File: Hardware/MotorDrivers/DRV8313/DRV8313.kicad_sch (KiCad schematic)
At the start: 61 parts, among them CN10 PR5L4015-5P-C-F, CN11 PR5L4015-5P-C-F, CN7 PR5L4015-5P-C-F, CN8 PR5L4015-5P-C-F, CN9 PR5L4015-5P-C-F, J1 Conn_01x04_Socket, J3 Conn_01x02_Socket, J4 Conn_01x03_Socket, Q1 BSS123_C427379, Q2 BSS123_C427379, U1 MS8313, U2 TLV9001IDCK, U35 PR5L5015-5P-C-H, U36 PR5L5015-5P-C-H, U37 PR5L5015-5P-C-H, U38 PR5L5015-5P-C-H, U39 PR5L5015-5P-C-H, U5 INA241A2xD, U6 INA241A2xD, U7 INA241A2xD

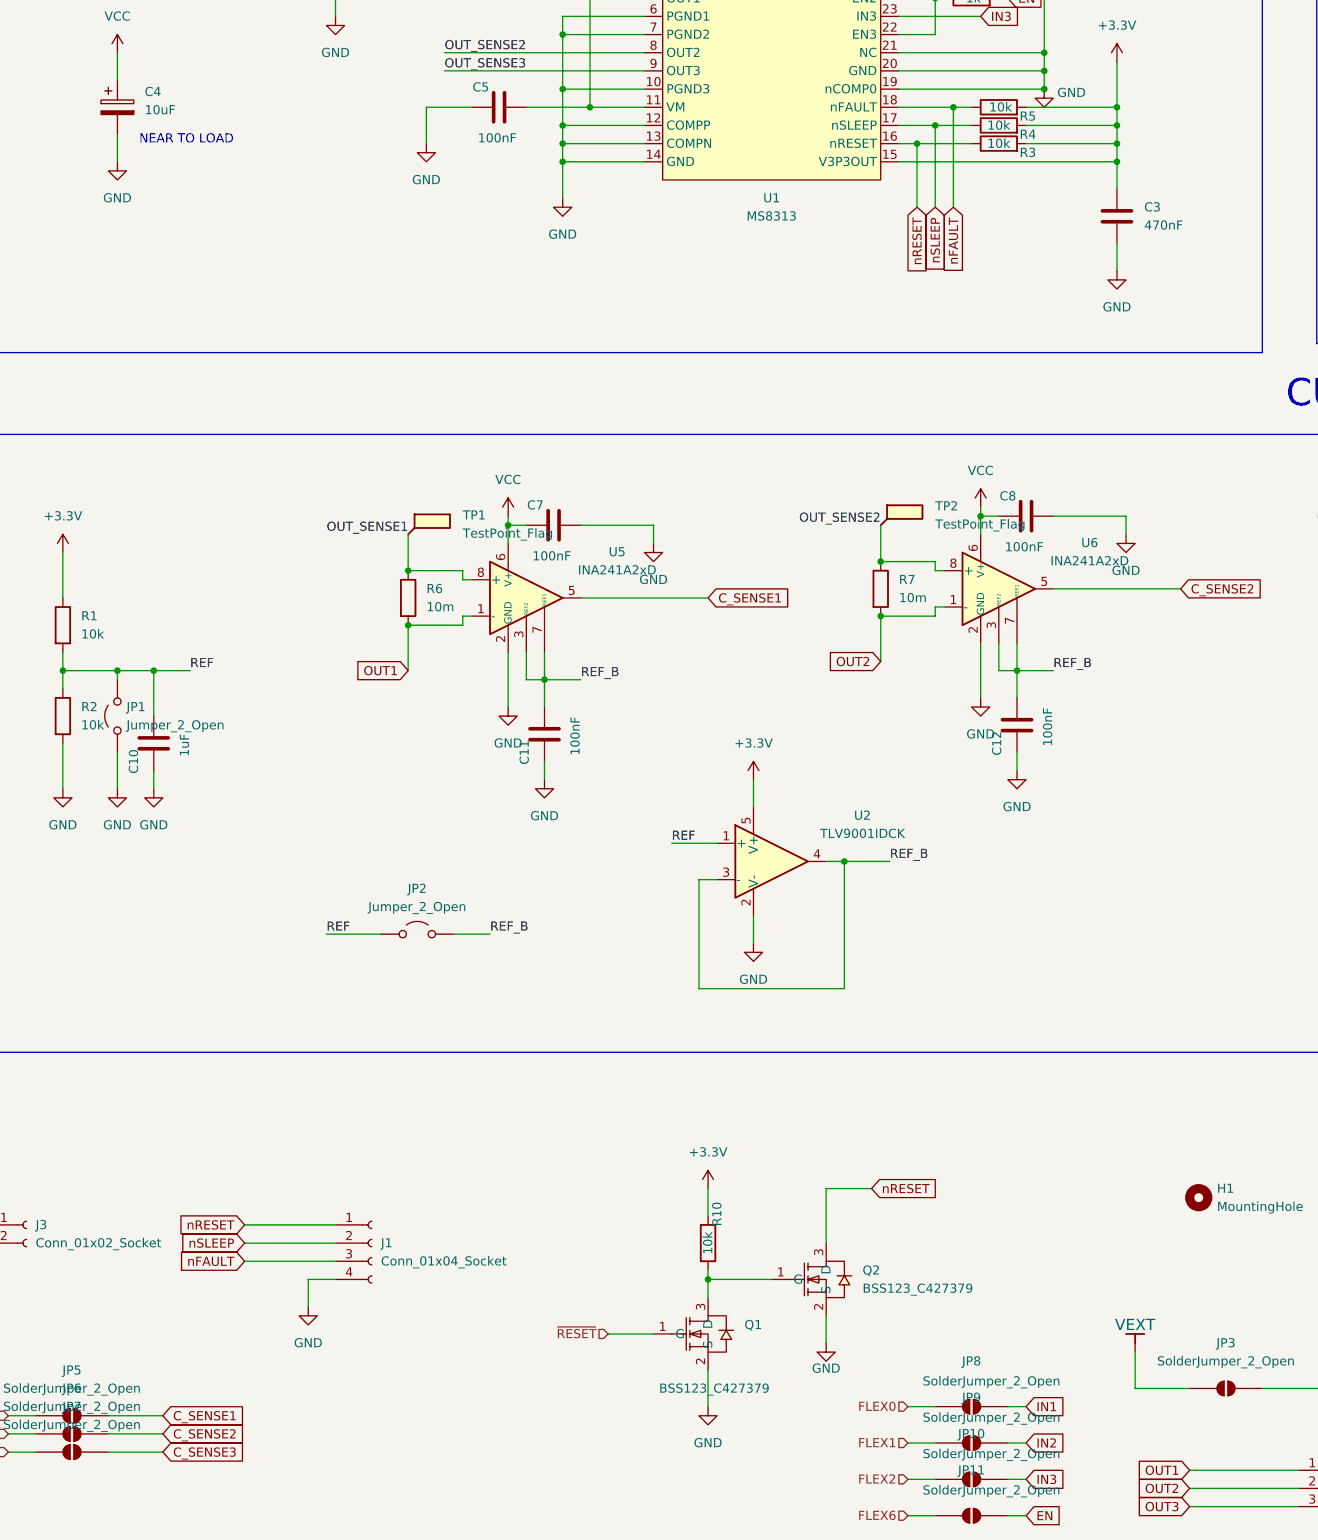
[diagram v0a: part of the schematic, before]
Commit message: placed components
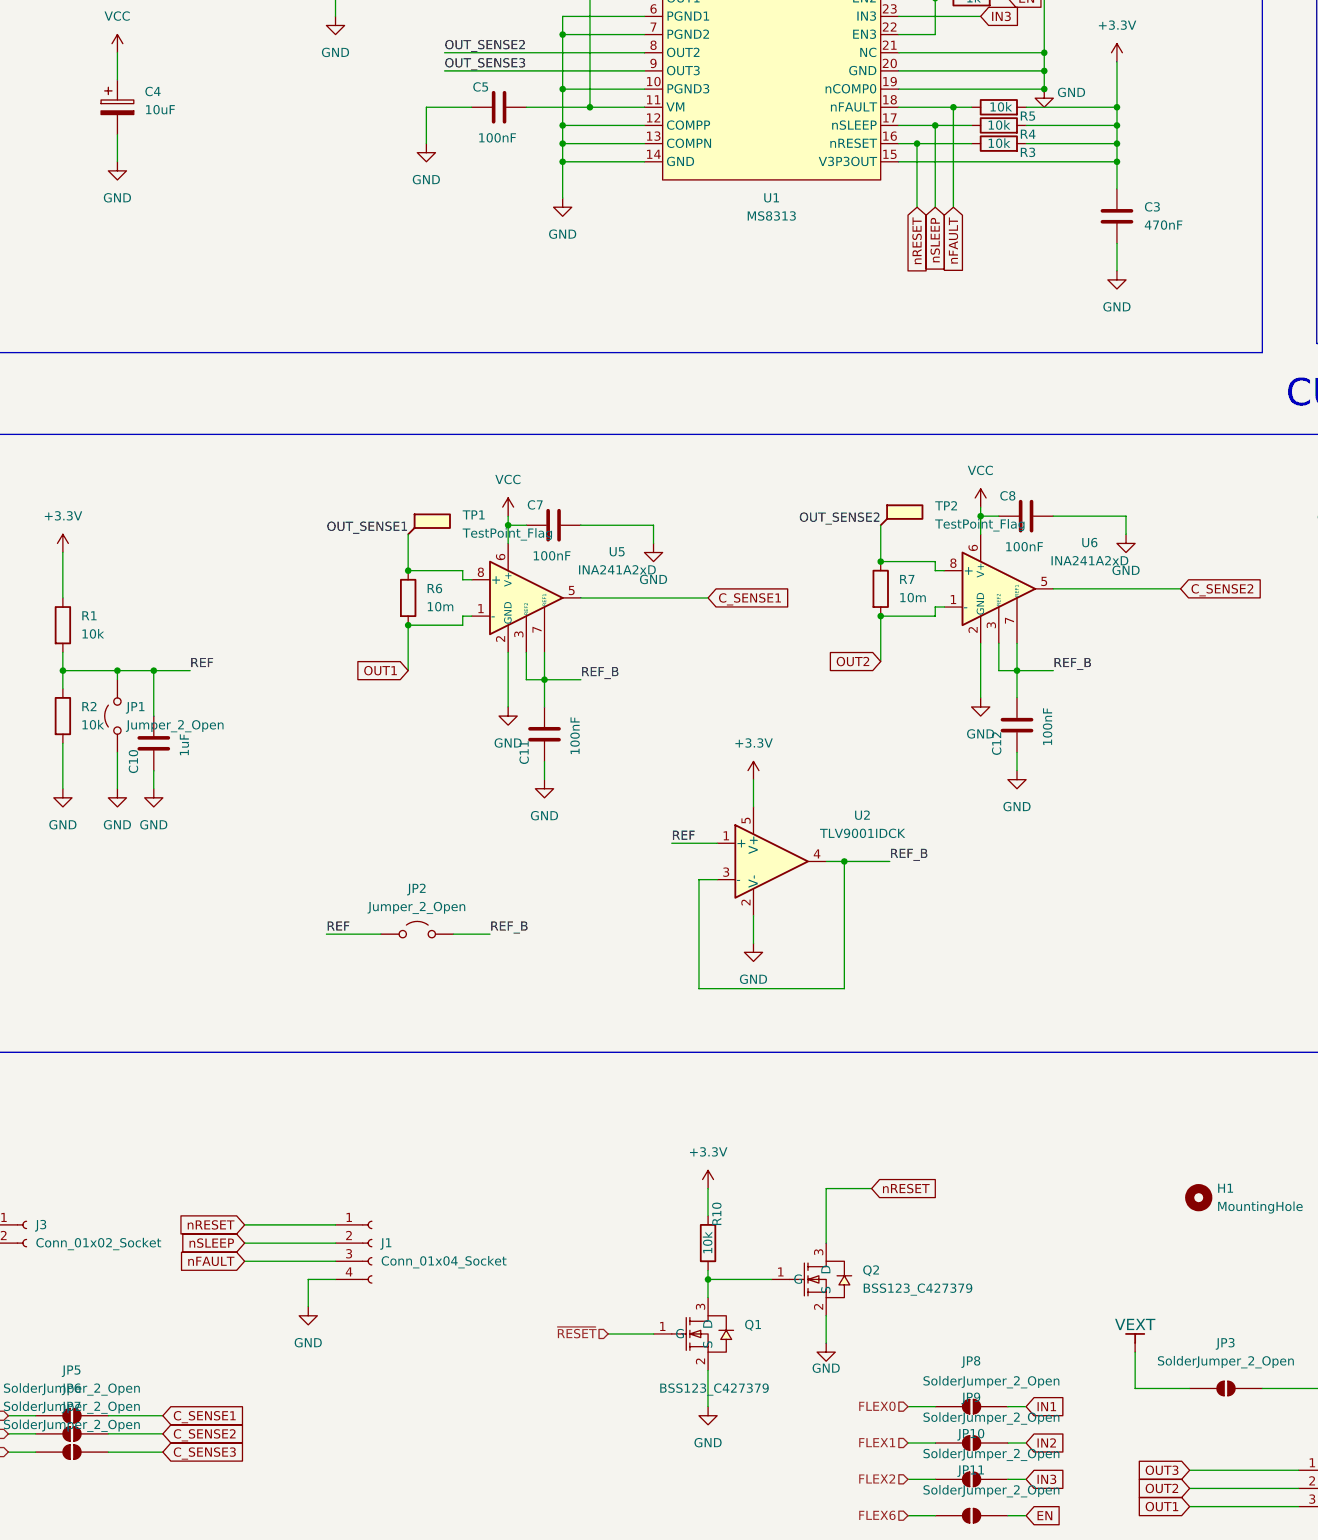
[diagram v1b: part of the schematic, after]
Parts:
- C4: footprint SpaghettiLAB:C0603 -> SpaghettiLAB:C1206
- J3: footprint Connector_PinSocket_1.27mm:PinSocket_1x03_P1.27mm_Vertical -> Connector_PinSocket_1.27mm:PinSocket_1x02_P1.27mm_Vertical
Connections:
- net OUT1: now also J4.3 (Pin_3); no longer J4.1 (Pin_1)
- net OUT3: now also J4.1 (Pin_1); no longer J4.3 (Pin_3)
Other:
- note removed: "NEAR TO LOAD"
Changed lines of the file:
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@@
 		)
 	)
-	(text "NEAR TO LOAD"
-		(exclude_from_sim no)
-		(at 64.262 87.122 0)
-		(effects
-			(font
-				(size 1.27 1.27)
-			)
-		)
-	)
 	(text "MOTOR DRIVER\n"
 		(exclude_from_sim no)
@@
 		)
 	)
-	(global_label "nFAULT"
+	(global_label "OUT1"
 		(shape input)
-		(at 72.39 243.84 180)
+		(at 204.47 278.13 180)
 		(fields_autoplaced yes)
 		(effects
@@
 		)
 		(property "Intersheetrefs" "${INTERSHEET_REFS}"
-			(at 62.7524 243.84 0)
+			(at 196.6467 278.13 0)
 			(hide yes)
 			(show_name no)
@@
 		)
 	)
-	(global_label "OUT1"
+	(global_label "nFAULT"
 		(shape input)
-		(at 204.47 273.05 180)
+		(at 72.39 243.84 180)
 		(fields_autoplaced yes)
 		(effects
@@
 		)
 		(property "Intersheetrefs" "${INTERSHEET_REFS}"
-			(at 196.6467 273.05 0)
+			(at 62.7524 243.84 0)
 			(hide yes)
 			(show_name no)
@@
 		)
 	)
-	(global_label "OUT3"
+	(global_label "C_SENSE2"
 		(shape input)
-		(at 204.47 278.13 180)
+		(at 203.2 149.86 0)
 		(fields_autoplaced yes)
 		(effects
@@
 				(size 1.27 1.27)
 			)
-			(justify right)
+			(justify left)
 		)
 		(property "Intersheetrefs" "${INTERSHEET_REFS}"
-			(at 196.6467 278.13 0)
+			(at 215.6798 149.86 0)
 			(hide yes)
 			(show_name no)
@@
 					(size 1.27 1.27)
 				)
-				(justify right)
+				(justify left)
 			)
 		)
 	)
-	(global_label "C_SENSE2"
+	(global_label "OUT3"
 		(shape input)
-		(at 203.2 149.86 0)
+		(at 204.47 273.05 180)
 		(fields_autoplaced yes)
 		(effects
@@
 				(size 1.27 1.27)
 			)
-			(justify left)
+			(justify right)
 		)
 		(property "Intersheetrefs" "${INTERSHEET_REFS}"
-			(at 215.6798 149.86 0)
+			(at 196.6467 273.05 0)
 			(hide yes)
 			(show_name no)
@@
 					(size 1.27 1.27)
 				)
-				(justify left)
+				(justify right)
 			)
 		)
@@
 			)
 		)
-		(property "Footprint" "SpaghettiLAB:C0603"
+		(property "Footprint" "SpaghettiLAB:C1206"
 			(at 55.5752 86.36 0)
 			(hide yes)
@@
 			)
 		)
-		(property "Footprint" "Connector_PinSocket_1.27mm:PinSocket_1x03_P1.27mm_Vertical"
+		(property "Footprint" "Connector_PinSocket_1.27mm:PinSocket_1x02_P1.27mm_Vertical"
 			(at 41.91 238.76 0)
 			(hide yes)
